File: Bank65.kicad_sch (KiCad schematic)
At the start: 2 parts, among them U1 XCKU5P-FFVB676

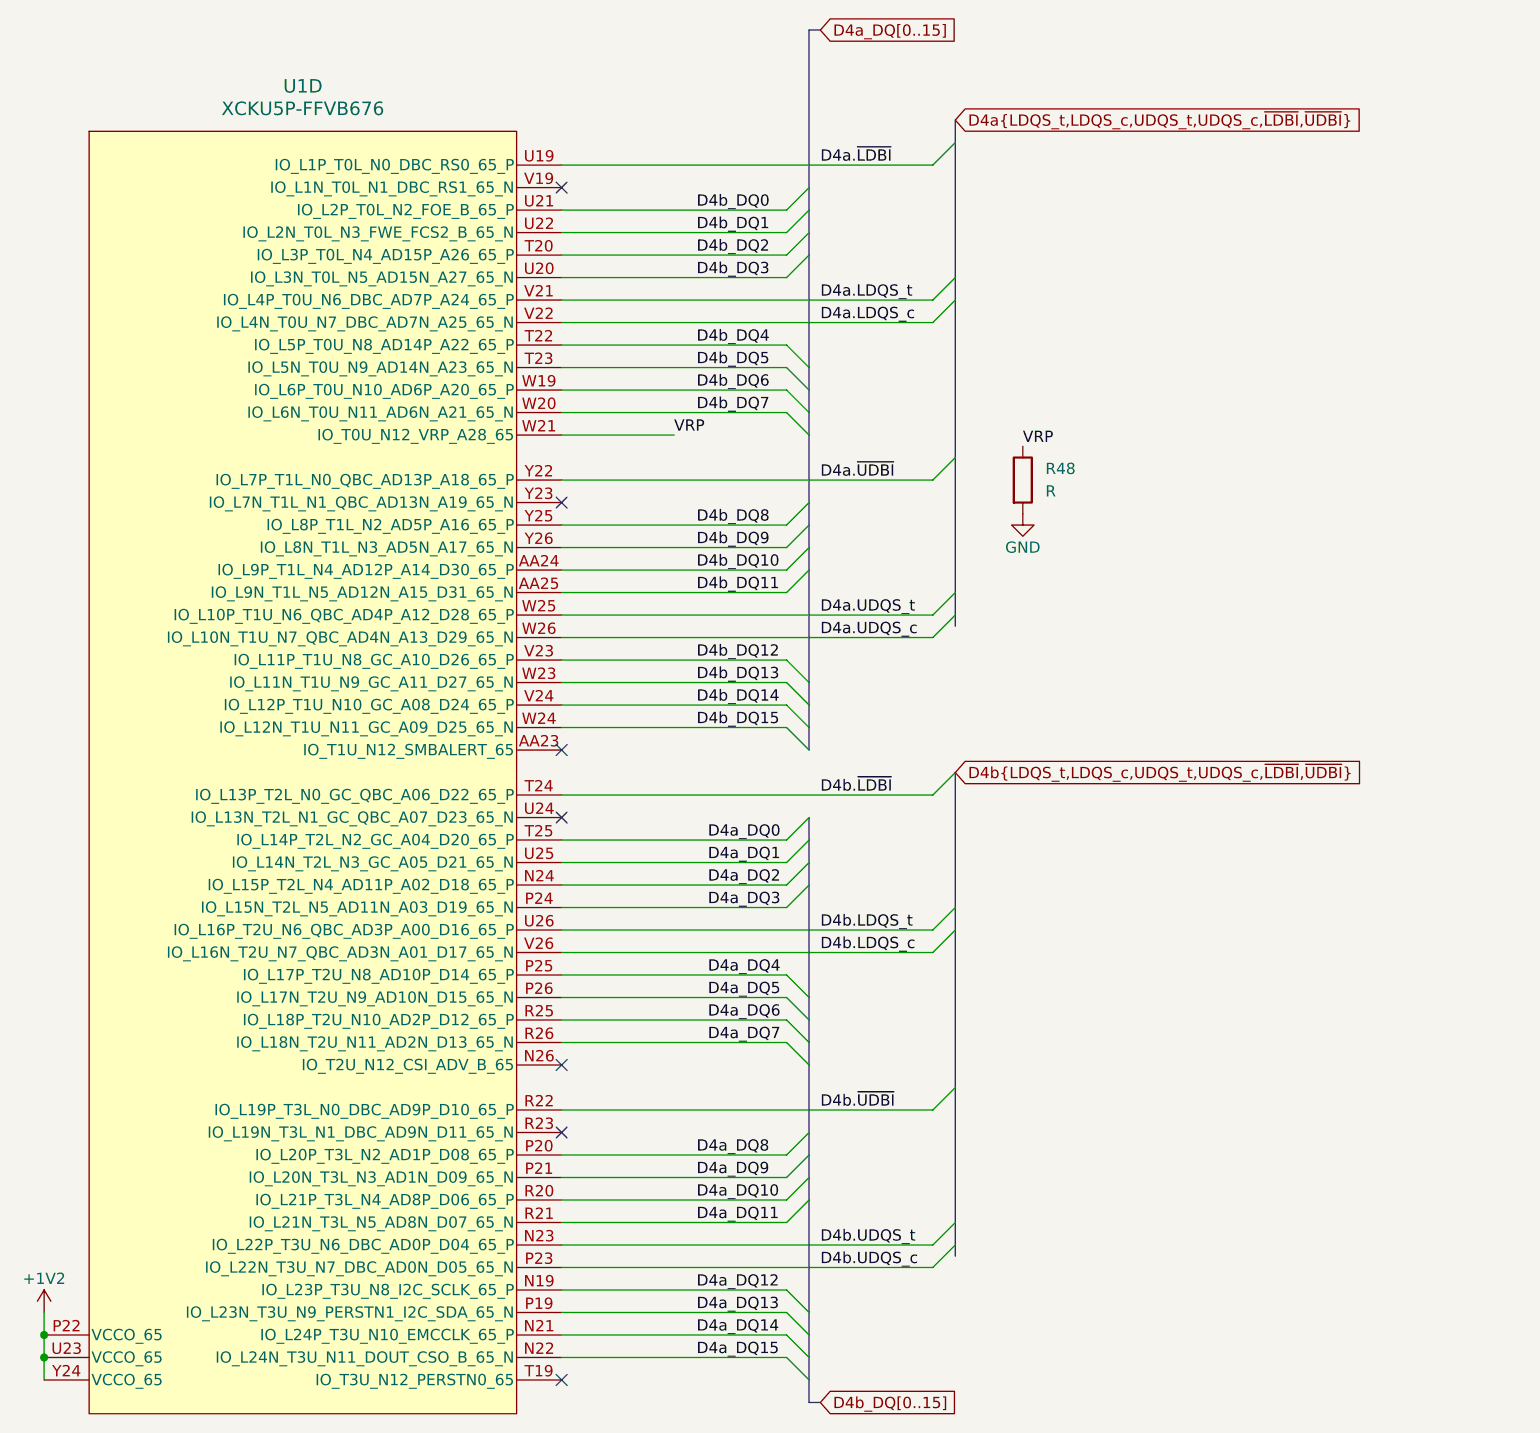
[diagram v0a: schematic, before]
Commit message: pushing the schematics works
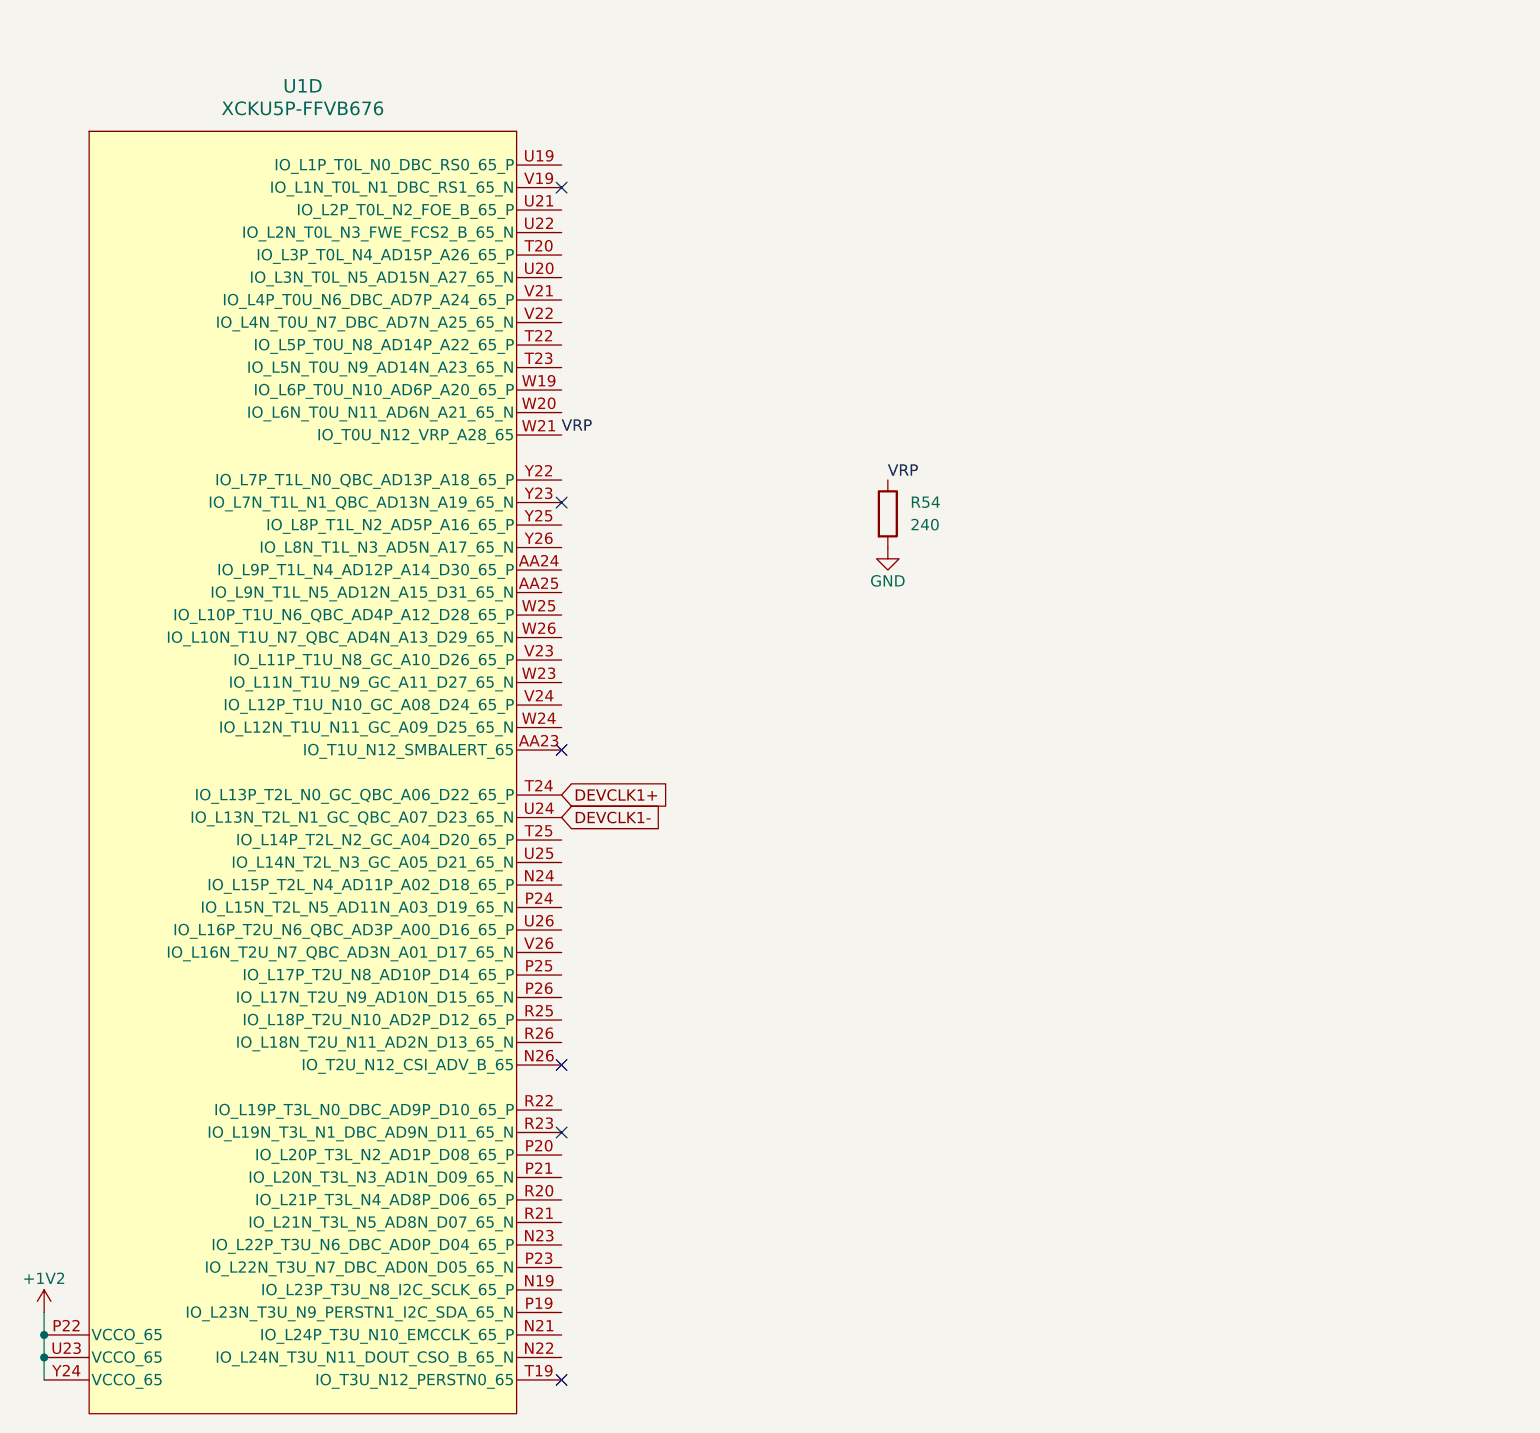
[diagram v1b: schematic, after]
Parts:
- removed R48: R, Resistor_SMD:R_0201_0603Metric, symbol Device:R
- added R54: 240, Resistor_SMD:R_0201_0603Metric, symbol Device:R
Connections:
- net GND: now also R54.2
- net VRP: now also R54.1
- net DEVCLK1-: now reaches U1.U24 (IO_L13N_T2L_N1_GC_QBC_A07_D23_65_N)
- net D4a.LDQS_c: no longer names the net of U1.V22 (IO_L4N_T0U_N7_DBC_AD7N_A25_65_N)
- net D4a.LDQS_t: no longer names the net of U1.V21 (IO_L4P_T0U_N6_DBC_AD7P_A24_65_P)
- net D4a.UDQS_c: no longer names the net of U1.W26 (IO_L10N_T1U_N7_QBC_AD4N_A13_D29_65_N)
- net D4a.UDQS_t: no longer names the net of U1.W25 (IO_L10P_T1U_N6_QBC_AD4P_A12_D28_65_P)
- net D4a.~{LDBI}: no longer names the net of U1.U19 (IO_L1P_T0L_N0_DBC_RS0_65_P)
- net D4a.~{UDBI}: no longer names the net of U1.Y22 (IO_L7P_T1L_N0_QBC_AD13P_A18_65_P)
- net D4a_DQ0: no longer names the net of U1.T25 (IO_L14P_T2L_N2_GC_A04_D20_65_P)
- net D4a_DQ1: no longer names the net of U1.U25 (IO_L14N_T2L_N3_GC_A05_D21_65_N)
- net D4a_DQ10: no longer names the net of U1.R20 (IO_L21P_T3L_N4_AD8P_D06_65_P)
- net D4a_DQ11: no longer names the net of U1.R21 (IO_L21N_T3L_N5_AD8N_D07_65_N)
- net D4a_DQ12: no longer names the net of U1.N19 (IO_L23P_T3U_N8_I2C_SCLK_65_P)
- net D4a_DQ13: no longer names the net of U1.P19 (IO_L23N_T3U_N9_PERSTN1_I2C_SDA_65_N)
- net D4a_DQ14: no longer names the net of U1.N21 (IO_L24P_T3U_N10_EMCCLK_65_P)
- net D4a_DQ15: no longer names the net of U1.N22 (IO_L24N_T3U_N11_DOUT_CSO_B_65_N)
- net D4a_DQ2: no longer names the net of U1.N24 (IO_L15P_T2L_N4_AD11P_A02_D18_65_P)
- net D4a_DQ3: no longer names the net of U1.P24 (IO_L15N_T2L_N5_AD11N_A03_D19_65_N)
- net D4a_DQ4: no longer names the net of U1.P25 (IO_L17P_T2U_N8_AD10P_D14_65_P)
- net D4a_DQ5: no longer names the net of U1.P26 (IO_L17N_T2U_N9_AD10N_D15_65_N)
- net D4a_DQ6: no longer names the net of U1.R25 (IO_L18P_T2U_N10_AD2P_D12_65_P)
- net D4a_DQ7: no longer names the net of U1.R26 (IO_L18N_T2U_N11_AD2N_D13_65_N)
- net D4a_DQ8: no longer names the net of U1.P20 (IO_L20P_T3L_N2_AD1P_D08_65_P)
- net D4a_DQ9: no longer names the net of U1.P21 (IO_L20N_T3L_N3_AD1N_D09_65_N)
- net D4b.LDQS_c: no longer names the net of U1.V26 (IO_L16N_T2U_N7_QBC_AD3N_A01_D17_65_N)
- net D4b.LDQS_t: no longer names the net of U1.U26 (IO_L16P_T2U_N6_QBC_AD3P_A00_D16_65_P)
- net D4b.UDQS_c: no longer names the net of U1.P23 (IO_L22N_T3U_N7_DBC_AD0N_D05_65_N)
- net D4b.UDQS_t: no longer names the net of U1.N23 (IO_L22P_T3U_N6_DBC_AD0P_D04_65_P)
- net D4b.~{LDBI} renamed DEVCLK1+
- net D4b.~{UDBI}: no longer names the net of U1.R22 (IO_L19P_T3L_N0_DBC_AD9P_D10_65_P)
- net D4b_DQ0: no longer names the net of U1.U21 (IO_L2P_T0L_N2_FOE_B_65_P)
- net D4b_DQ1: no longer names the net of U1.U22 (IO_L2N_T0L_N3_FWE_FCS2_B_65_N)
- net D4b_DQ10: no longer names the net of U1.AA24 (IO_L9P_T1L_N4_AD12P_A14_D30_65_P)
- net D4b_DQ11: no longer names the net of U1.AA25 (IO_L9N_T1L_N5_AD12N_A15_D31_65_N)
- net D4b_DQ12: no longer names the net of U1.V23 (IO_L11P_T1U_N8_GC_A10_D26_65_P)
- net D4b_DQ13: no longer names the net of U1.W23 (IO_L11N_T1U_N9_GC_A11_D27_65_N)
- net D4b_DQ14: no longer names the net of U1.V24 (IO_L12P_T1U_N10_GC_A08_D24_65_P)
- net D4b_DQ15: no longer names the net of U1.W24 (IO_L12N_T1U_N11_GC_A09_D25_65_N)
- net D4b_DQ2: no longer names the net of U1.T20 (IO_L3P_T0L_N4_AD15P_A26_65_P)
- net D4b_DQ3: no longer names the net of U1.U20 (IO_L3N_T0L_N5_AD15N_A27_65_N)
- net D4b_DQ4: no longer names the net of U1.T22 (IO_L5P_T0U_N8_AD14P_A22_65_P)
- net D4b_DQ5: no longer names the net of U1.T23 (IO_L5N_T0U_N9_AD14N_A23_65_N)
- net D4b_DQ6: no longer names the net of U1.W19 (IO_L6P_T0U_N10_AD6P_A20_65_P)
- net D4b_DQ7: no longer names the net of U1.W20 (IO_L6N_T0U_N11_AD6N_A21_65_N)
- net D4b_DQ8: no longer names the net of U1.Y25 (IO_L8P_T1L_N2_AD5P_A16_65_P)
- net D4b_DQ9: no longer names the net of U1.Y26 (IO_L8N_T1L_N3_AD5N_A17_65_N)
- no-connect marks 7 -> 6
